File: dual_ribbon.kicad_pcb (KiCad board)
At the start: 2 copper layers, 100.5 x 101 mm, 52 parts, among them J1 Conn_01x02_Socket, J2 Conn_01x02_Socket, J3 Conn_01x02_Socket, J4 Conn_01x02_Socket, Q1 PNP, Q2 MMBF4391, Q3 MMBF4391, U1 LM4041LP-ADJ, U2 TL072, U3 OPA2134, U4 TL072, U5 TL072

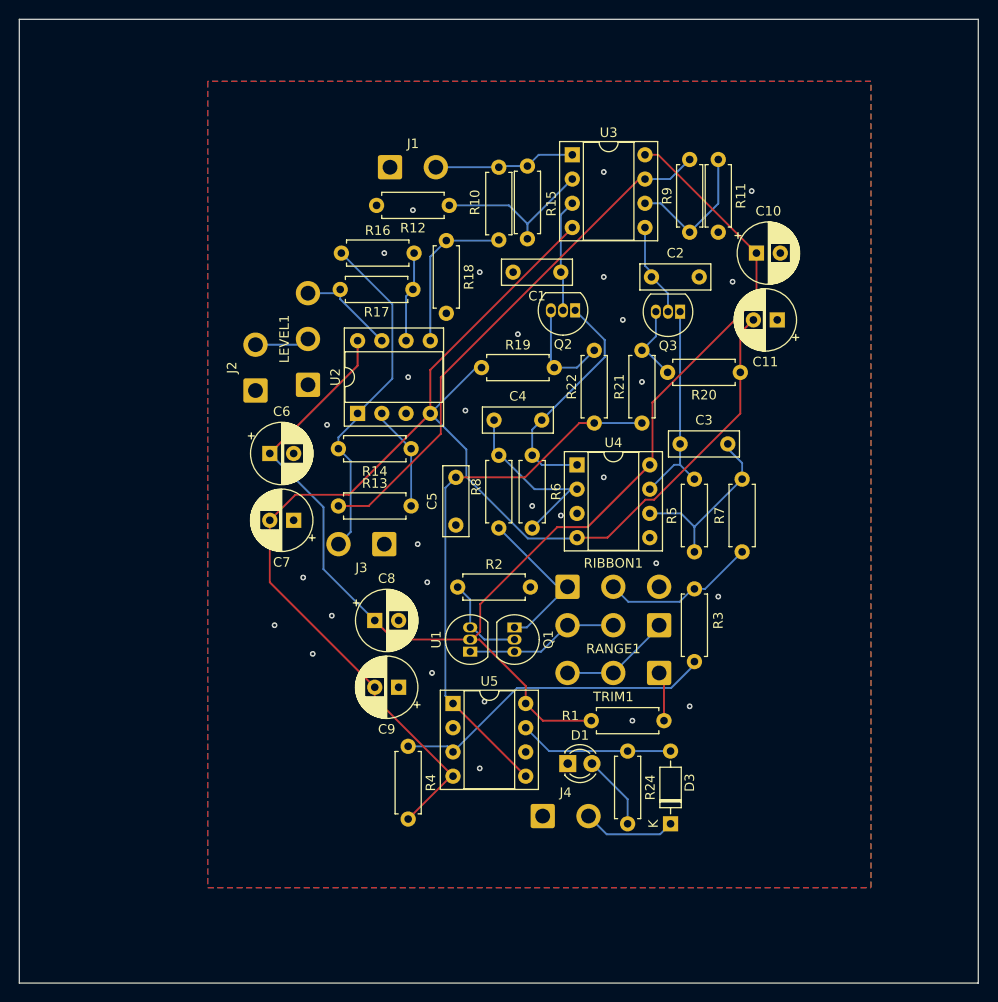
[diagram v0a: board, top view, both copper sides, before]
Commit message: Do gerbers
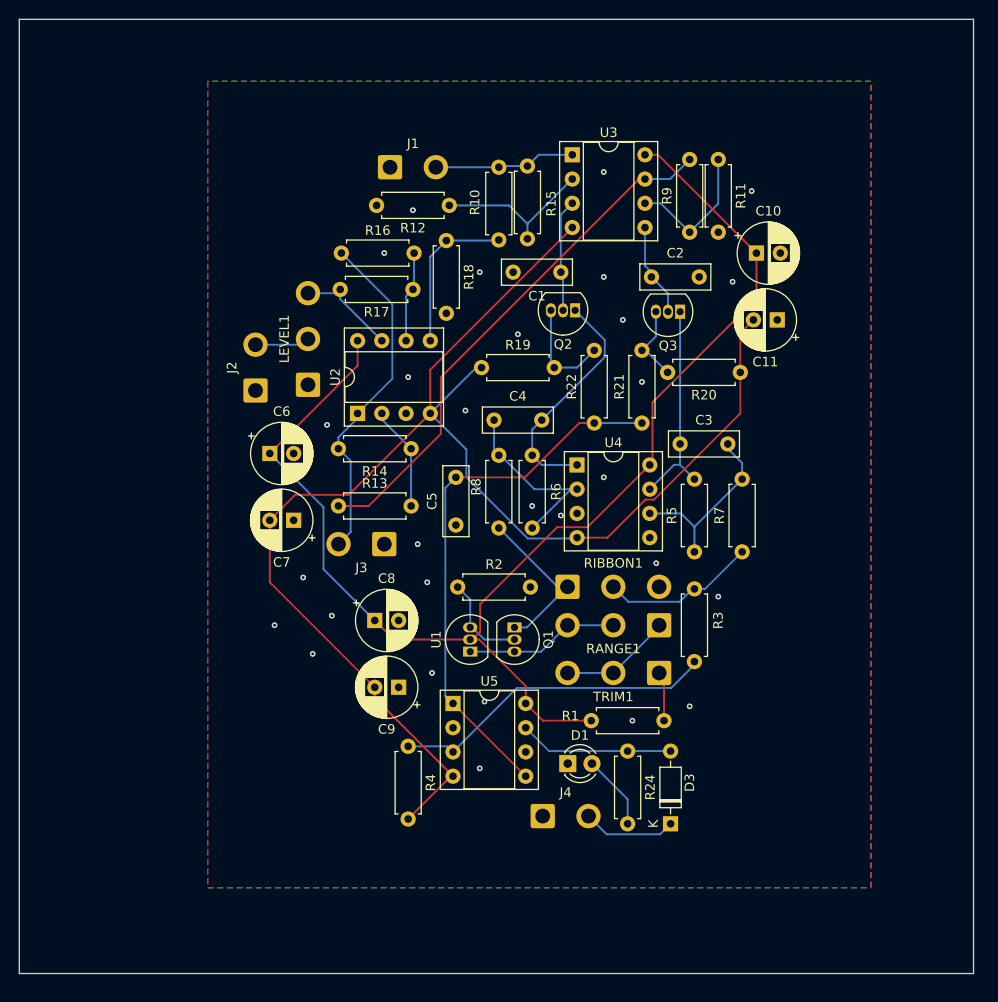
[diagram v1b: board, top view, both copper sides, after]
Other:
- board size 100.5 x 101 mm -> 100 x 100 mm
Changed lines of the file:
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@@
 			(outputformat 1)
 			(mirror no)
-			(drillshape 1)
+			(drillshape 0)
 			(scaleselection 1)
-			(outputdirectory "")
+			(outputdirectory "C:/Users/nolan.greig/Documents/flerb/")
 		)
 	)
@@
 	(gr_rect
 		(start 110.75 38.5)
-		(end 211.25 139.5)
+		(end 210.75 138.5)
 		(stroke
 			(width 0.05)
